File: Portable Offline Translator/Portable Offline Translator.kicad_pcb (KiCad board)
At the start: 2 copper layers, 51 parts, among them J201 Conn_01x08_Male, J301 Conn_02x03_Odd_Even, SW301 SW_Push, SW302 SW_Push, SW303 SW_Push, SW304 SW_Push, U201 MAX98357AEWL+T, U301 STM32F407IEHx, U401 LM317_SOT-223, U402 LM317_SOT-223, Y301 Crystal

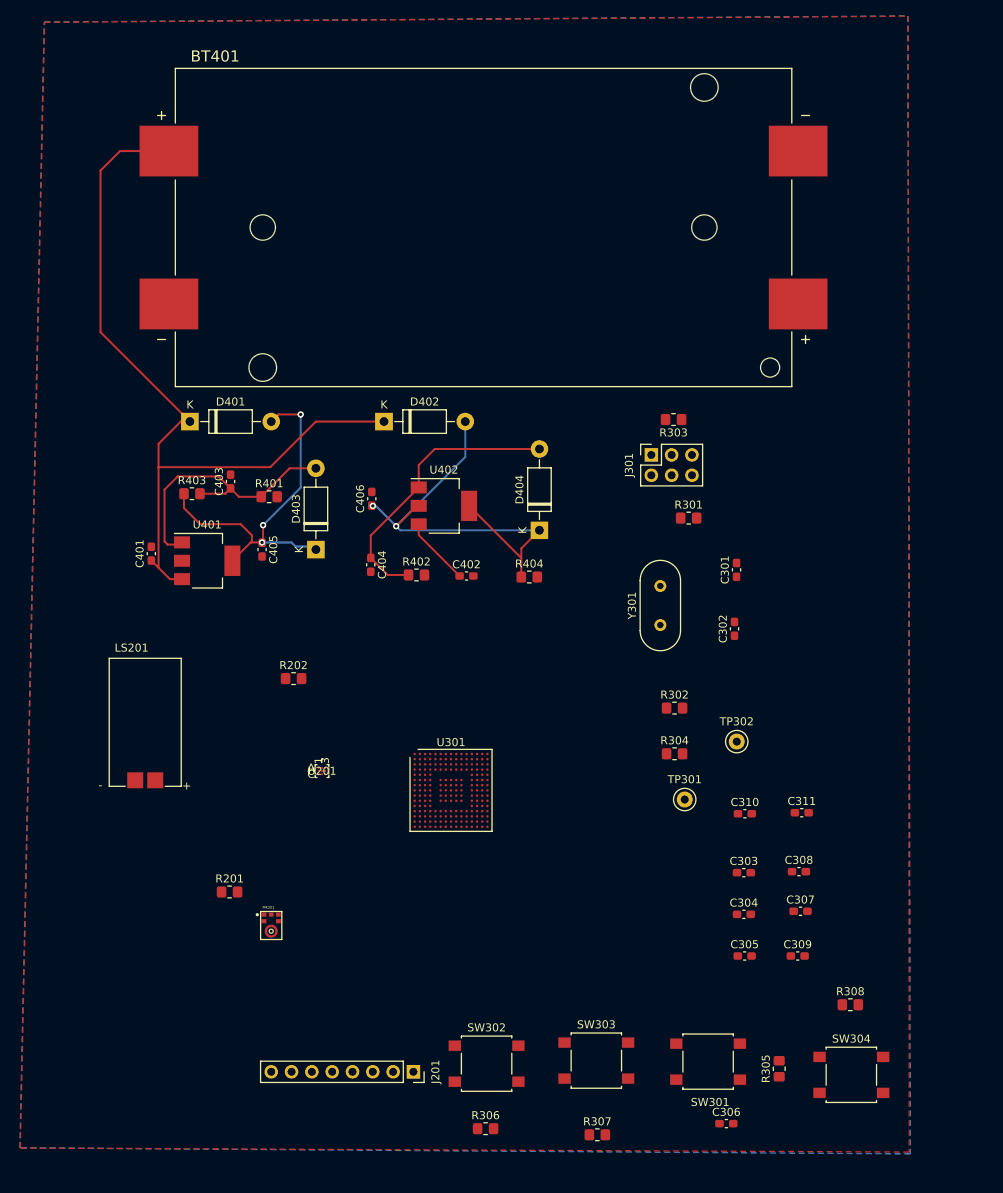
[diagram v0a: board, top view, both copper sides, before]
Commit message: PCB iteration 1
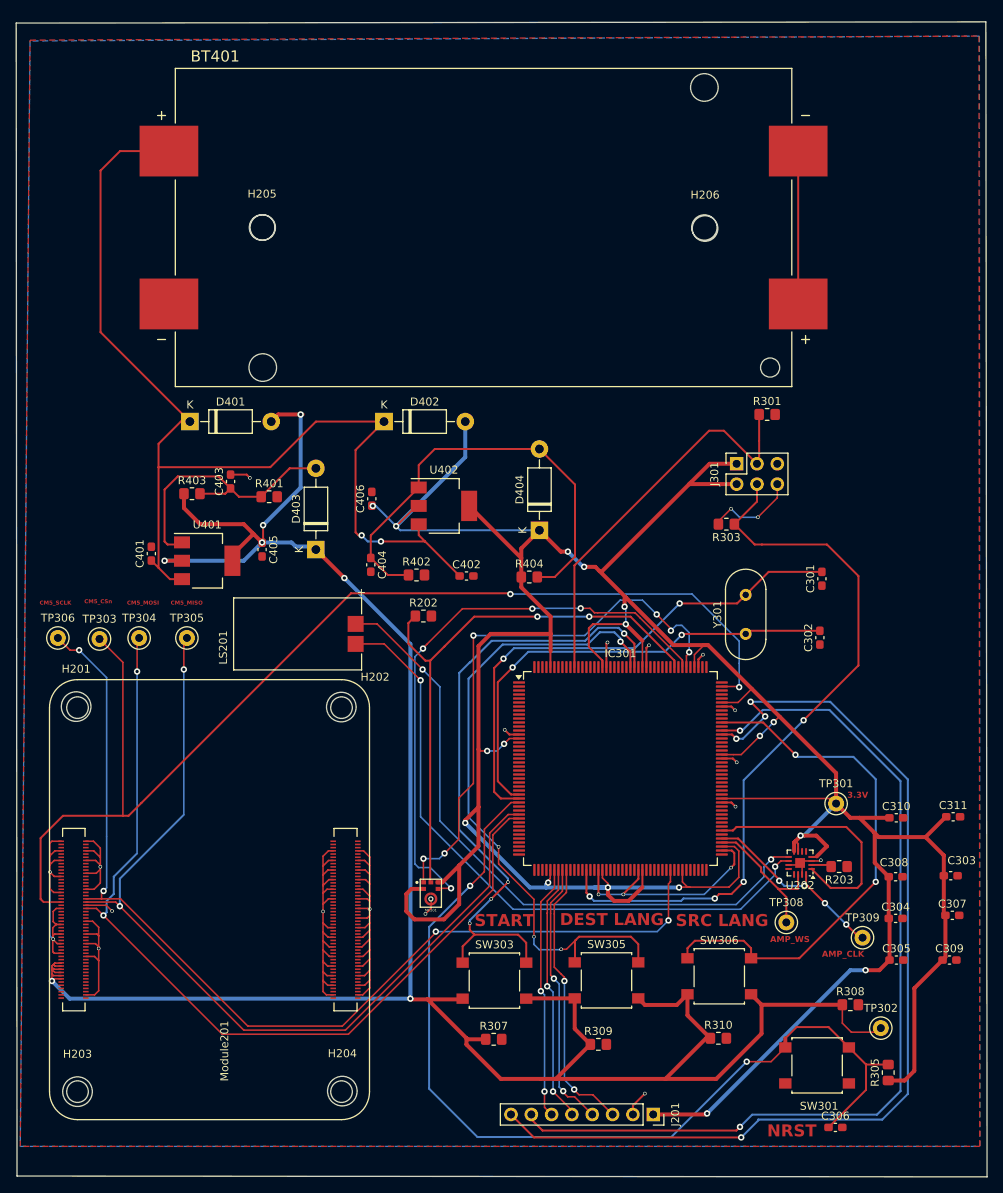
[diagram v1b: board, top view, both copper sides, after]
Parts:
- removed R201: 100k, Resistor_SMD:R_0805_2012Metric_Pad1.20x1.40mm_HandSolder
- removed R302, R304: 2k2, Resistor_SMD:R_0805_2012Metric_Pad1.20x1.40mm_HandSolder
- removed R306: 10k, Resistor_SMD:R_0805_2012Metric_Pad1.20x1.40mm_HandSolder
- removed SW302, SW304: SW_Push, Button_Switch_SMD:SW_SPST_B3S-1000
- removed U201: MAX98357AEWL+T, MAX98357AEWL_T(Audio Amp):21-0896B_9_MXM
- removed U301: STM32F407IEHx, Package_BGA:UFBGA-201_10x10mm_Layout15x15_P0.65mm
- added H201: MountingHole, MountingHole:MountingHole_3.7mm, F.Cu at (85.2, 99.5)
- added H202: MountingHole, MountingHole:MountingHole_3.7mm, F.Cu at (118.4, 99.6)
- added H203: MountingHole, MountingHole:MountingHole_3.7mm, F.Cu at (85.4, 147.6)
- added H204: MountingHole, MountingHole:MountingHole_3.7mm, F.Cu at (118.5, 147.6)
- added H205: MountingHole, MountingHole:MountingHole_3.2mm_M3, F.Cu at (108.5, 39.6)
- added H206: MountingHole, MountingHole:MountingHole_3.2mm_M3, F.Cu at (163.8, 39.8)
- added IC301: STM32F407IET6, Package_QFP:LQFP-176_24x24mm_P0.5mm, F.Cu at (153.3, 107.2)
- added Module201: ComputeModule5-CM5, CM5IO:Raspberry-Pi-5-Compute-Module, F.Cu at (85.4, 147.6)
- added R203: 100k, Resistor_SMD:R_0805_2012Metric_Pad1.20x1.40mm_HandSolder, F.Cu at (180.6, 119.5)
- added R309: 10k, Resistor_SMD:R_0805_2012Metric_Pad1.20x1.40mm_HandSolder, F.Cu at (150.5, 141.7)
- added R310: 10k, Resistor_SMD:R_0805_2012Metric_Pad1.20x1.40mm_HandSolder, F.Cu at (165.5, 141.0)
- added SW305: SW_Push, Button_Switch_SMD:SW_SPST_B3S-1000, F.Cu at (151.5, 133.7)
- added SW306: SW_Push, Button_Switch_SMD:SW_SPST_B3S-1000, F.Cu at (165.6, 133.2)
- added TP303: SPI4_CSn, TestPoint:TestPoint_Keystone_5000-5004_Miniature, F.Cu at (88.1, 91.1)
- added TP304: SPI4_MOSI, TestPoint:TestPoint_Keystone_5000-5004_Miniature, F.Cu at (93.1, 90.9)
- added TP305: SPI4_MISO, TestPoint:TestPoint_Keystone_5000-5004_Miniature, F.Cu at (99.1, 90.9)
- added TP306: SPI4_SCLK, TestPoint:TestPoint_Keystone_5000-5004_Miniature, F.Cu at (82.9, 90.9)
- added TP308: I2S_CLK, TestPoint:TestPoint_Keystone_5000-5004_Miniature, F.Cu at (174.0, 126.5)
- added TP309: 3.3V, TestPoint:TestPoint_Keystone_5000-5004_Miniature, F.Cu at (183.5, 128.4)
- added U202: MAX98357AETE_T, Package_DFN_QFN:TQFN-16-1EP_3x3mm_P0.5mm_EP1.23x1.23mm, F.Cu at (175.7, 119.1)
- TP302: value GND -> 5V
- moved TP302 40.1 mm to (185.8, 139.7)
- moved J201 30.4 mm to (157.4, 150.5)
- moved LS201 22.0 mm to (112.9, 90.4), turned to 90 degrees
- moved MK201 20.4 mm to (129.6, 122.8)
- moved C305 19.0 mm to (187.8, 131.2)
- moved C303 19.0 mm to (187.7, 120.8)
- moved C304 19.0 mm to (187.7, 126.0)
- moved C307 19.0 mm to (194.7, 125.6)
- moved C308 19.0 mm to (194.5, 120.7)
- moved C309 19.0 mm to (194.4, 131.2)
- moved C311 18.9 mm to (194.8, 113.3)
- moved TP301 18.9 mm to (180.2, 111.6)
- moved C310 18.9 mm to (187.7, 113.4)
- moved R202 18.0 mm to (128.6, 88.2)
- moved R307 17.6 mm to (137.4, 141.1)
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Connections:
- net OSC_IN renamed /MCU/OSC_IN
- net OSC_OUT renamed /MCU/OSC_OUT
- C303 pad 1: +3V3 -> +3.3V
- C304 pad 1: +3V3 -> +3.3V
- C305 pad 1: +3V3 -> +3.3V
- C307 pad 1: +3V3 -> +3.3V
- C308 pad 1: +3V3 -> +3.3V
- C309 pad 1: +3V3 -> +3.3V
- C310 pad 1: +3V3 -> +3.3V
- C311 pad 1: +3V3 -> +3.3V
- J201 pad 1: /IO Circuits/LCD_VCC -> +3.3V
- J201 pad 3: /IO Circuits/SPI_MISO -> /IO Circuits/SPI1_MOSI
- J201 pad 4: /IO Circuits/SPI1_SCK -> /IO Circuits/SPI_MISO
- J201 pad 5: /IO Circuits/SPI1_MOSI -> /IO Circuits/SPI1_SCK
- J301 pad 1: +3V3 -> +3.3V
- J301 pad 2: +3V3 -> +3.3V
- J301 pad 4: Net-(J301-Pad4) -> BOOT1
- R303 pad 1: Net-(J301-Pad4) -> BOOT1
- R305 pad 1: +3V3 -> +3.3V
- TP301 pad 1: +3V3 -> +3.3V
- TP302 pad 1: GND -> +5V
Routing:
- net +3.3V: track 58.6 -> 461.0 mm, vias 2 -> 17
- net +5V: track 46.8 -> 300.0 mm, vias 1 -> 7
- net GND: track 0.00 -> 221.1 mm, vias 2 -> 23
- net /IO Circuits/SPI4_CSn: track 0.00 -> 144.3 mm, vias 0 -> 2
- net /IO Circuits/SPI4_SCLK: track 0.00 -> 127.5 mm, vias 0 -> 4
- net /IO Circuits/LCD_RST: track 0.00 -> 125.5 mm, vias 0 -> 4
- net /MCU/NRST: track 0.00 -> 119.0 mm, vias 0 -> 2
- net /IO Circuits/LCD_Data/Command: track 0.00 -> 115.2 mm, vias 0 -> 2
- net /IO Circuits/SPI4_MISO: track 0.00 -> 112.8 mm, vias 0 -> 2
- net /IO Circuits/SPI4_MOSI: track 0.00 -> 112.4 mm, vias 0 -> 2
- net BOOT1: track 0.00 -> 92.5 mm, vias 0 -> 4
- net Net-(IC301-PG9): track 0.00 -> 82.0 mm, vias 0 -> 4
- net /IO Circuits/OUTP: track 0.00 -> 81.7 mm, vias 0 -> 2
- net /IO Circuits/OUTN: track 0.00 -> 81.0 mm, vias 0 -> 2
- net Net-(IC301-PD7): track 0.00 -> 78.9 mm, vias 0 -> 4
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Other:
- board outline added: 121.4 x 144.4 mm
- board text added: "3.3V"
- board text added: "AMP_CLK"
- board text added: "AMP_WS"
- board text added: "CM5_CSn"
- board text added: "CM5_MISO"
- board text added: "CM5_MOSI"
- board text added: "CM5_SCLK"
- board text added: "DEST LANG"
- board text added: "NRST"
- board text added: "SRC LANG"
- board text added: "START"
